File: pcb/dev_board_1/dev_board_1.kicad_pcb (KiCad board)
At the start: 2 copper layers, 91.5 x 93.5 mm, 76 parts, among them J1 Conn_01x03, P1 USB_C_Plug_USB2.0, SW1 SW_DIP_x01, SW10 SW_DIP_x01, SW11 SW_DIP_x01, SW12 SW_DIP_x01, SW13 SW_DIP_x01, SW14 SW_DIP_x01, SW15 SW_DIP_x01, SW16 SW_DIP_x01, SW17 SW_DIP_x01, SW18 SW_DIP_x01, SW19 SW_DIP_x01, SW2 SW_DIP_x01, SW20 SW_DIP_x01, SW21 SW_DIP_x01, SW22 SW_DIP_x01, SW23 SW_DIP_x01, SW24 SW_DIP_x01, SW3 SW_DIP_x01, SW4 SW_DIP_x01, SW5 SW_DIP_x01, SW6 SW_DIP_x01, SW7 SW_DIP_x01, SW8 SW_DIP_x01, SW9 SW_DIP_x01, U2 LD3985M33R_SOT23, U6 STM32F427ZGTx, U7 MT48LC16M16A2TG, Y1 Crystal

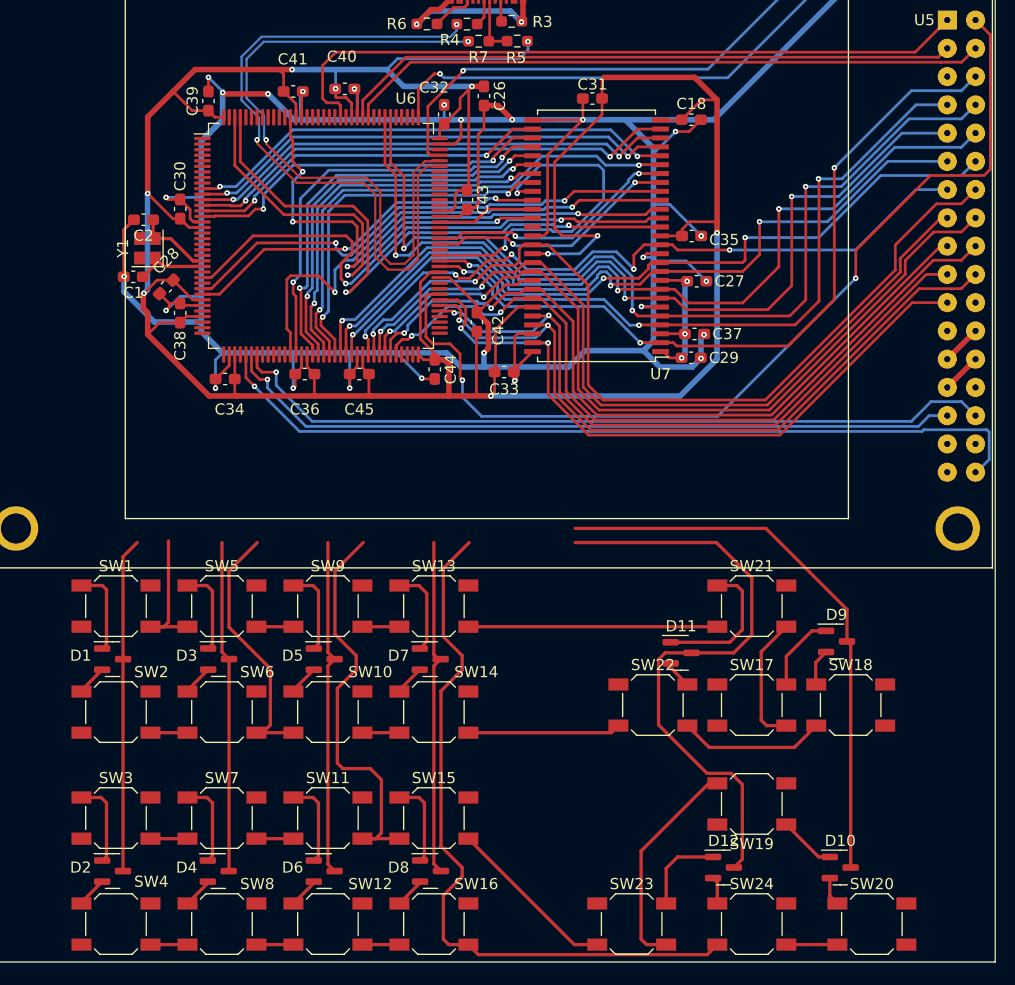
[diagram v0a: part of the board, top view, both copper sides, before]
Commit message: place buttons
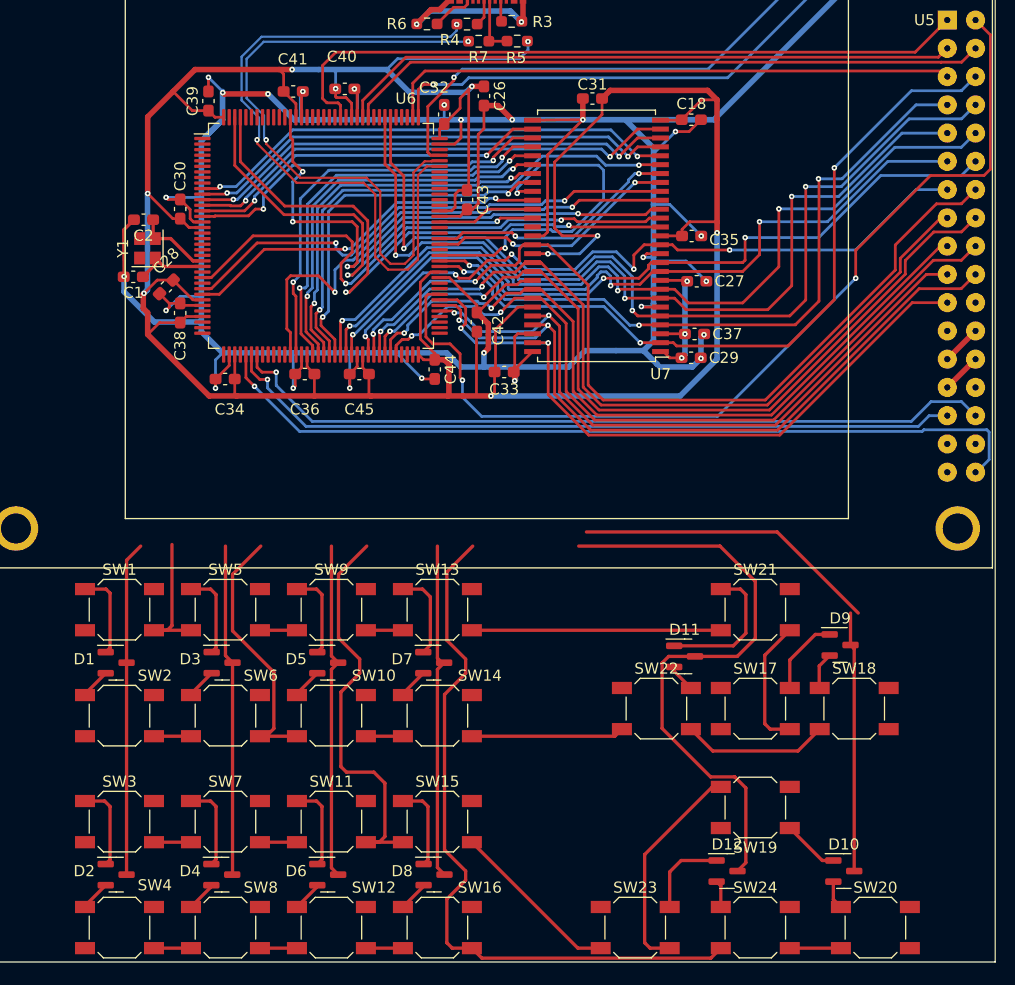
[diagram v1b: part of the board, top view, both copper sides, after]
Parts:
- moved D11 0.45 mm to (99.4, 84.8)
- moved D12 0.45 mm to (103.3, 104.1)
- moved D5 0.45 mm to (67.4, 85.4)
- moved D6 0.45 mm to (67.4, 104.4)
- moved D1 0.45 mm to (48.4, 85.4)
- moved D2 0.45 mm to (48.4, 104.4)
- moved D3 0.45 mm to (57.9, 85.3)
- moved D4 0.45 mm to (57.8, 104.4)
- moved SW5 0.45 mm to (58.2, 80.6)
- moved SW6 0.45 mm to (58.2, 90.1)
- moved SW7 0.45 mm to (58.2, 99.6)
- moved SW8 0.45 mm to (58.2, 109.2)
- moved D10 0.45 mm to (113.8, 104.1)
- moved D7 0.45 mm to (76.9, 85.4)
- moved D8 0.45 mm to (76.9, 104.4)
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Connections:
- U6 pad 110: unconnected-(U6-PA15-Pad110) -> /LCD_RESET
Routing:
- net /LCD_RESET: track 0.00 -> 51.8 mm
- net +3.3V: track 310.1 -> 308.5 mm
